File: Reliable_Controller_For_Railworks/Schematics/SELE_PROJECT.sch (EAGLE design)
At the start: 21 parts, among them IC1 24LC1025, IC2 MAX232, U1 328P, U2 LTC485N, U3 LTC485N, X1 16MHz

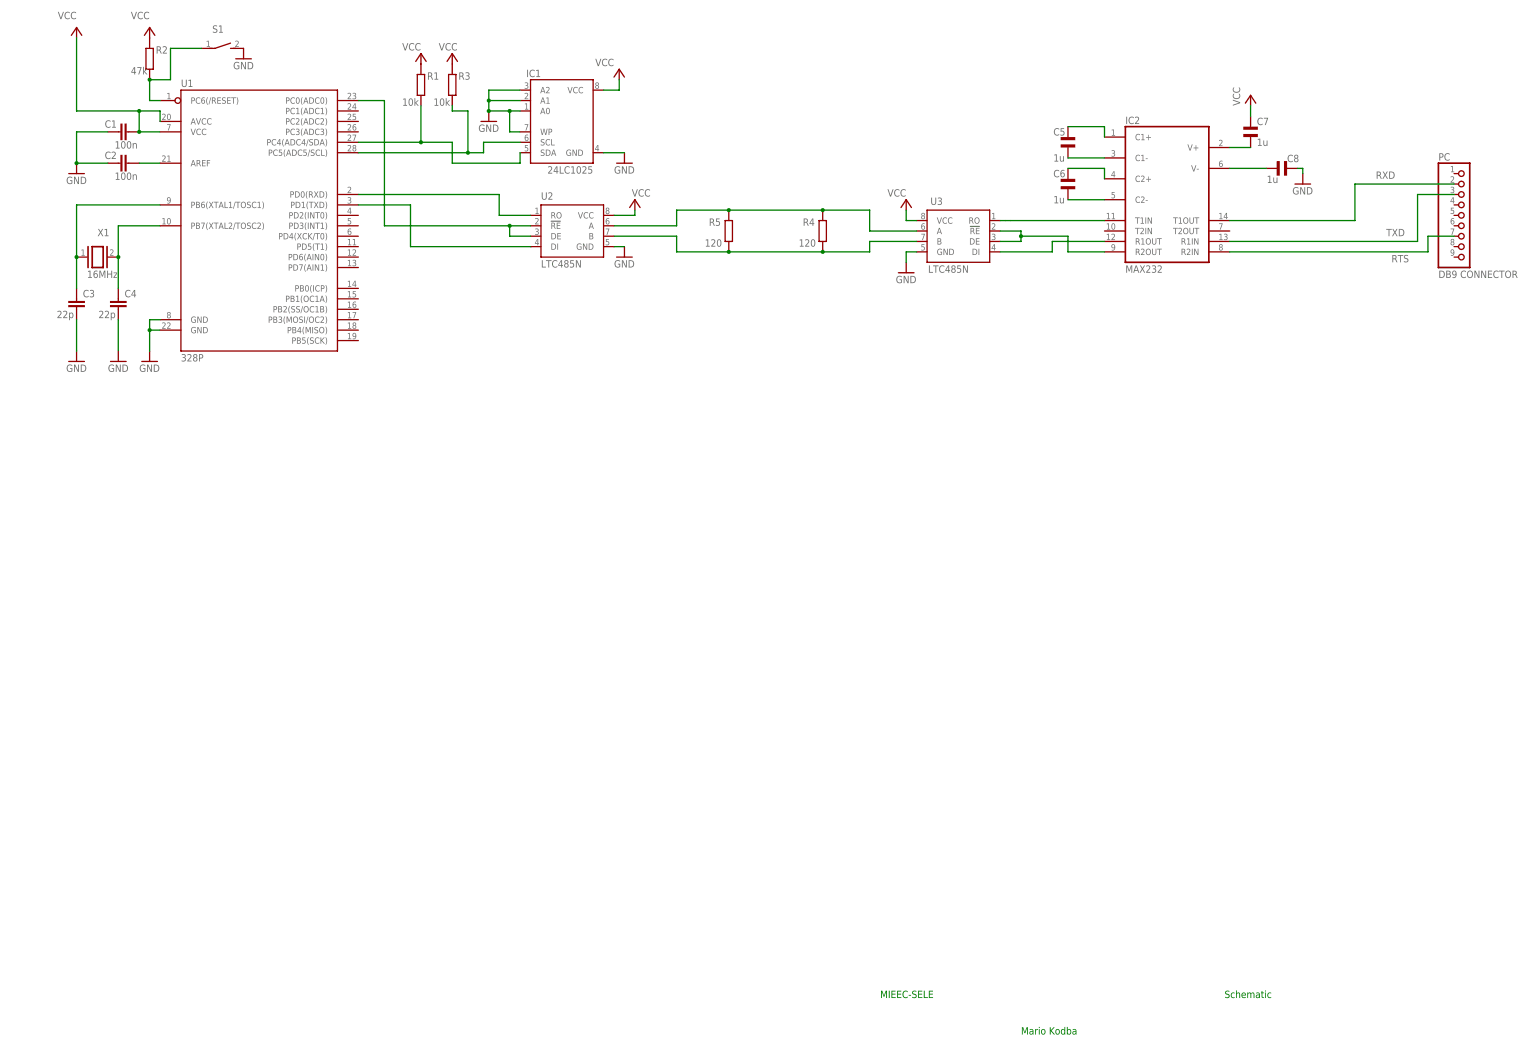
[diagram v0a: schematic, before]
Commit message: updated electrical schematic
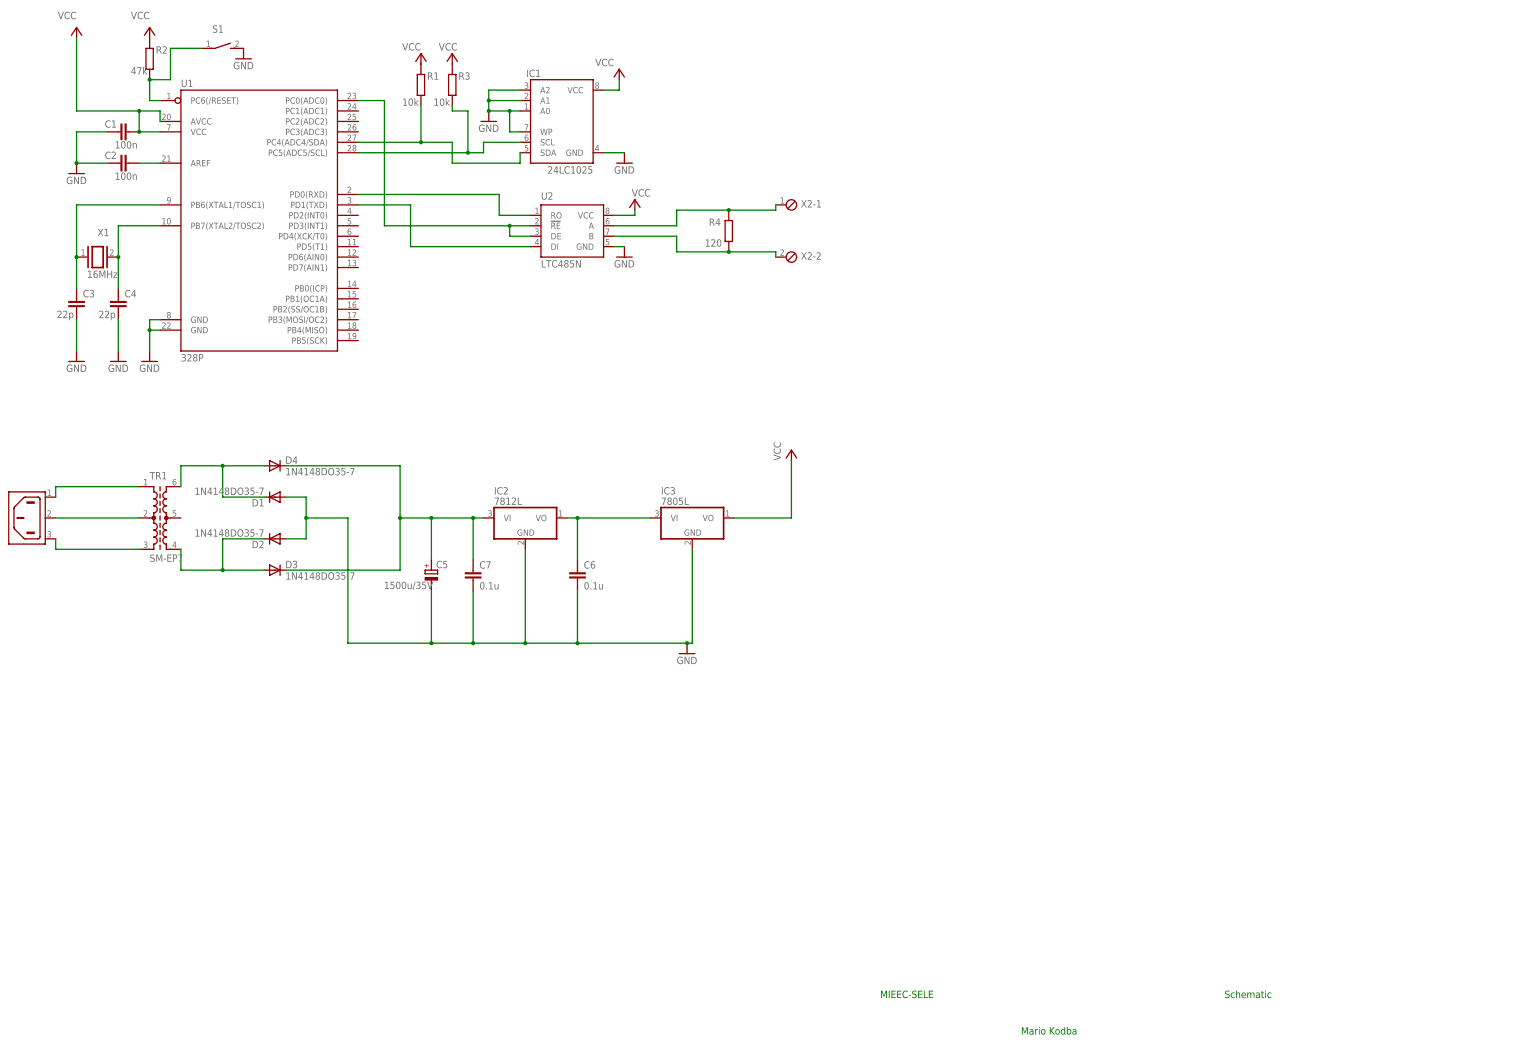
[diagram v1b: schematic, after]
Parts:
- removed C8: 1u, rcl:EL-BI25-10AXIAL
- removed PC: DB9 CONNECTOR, pinhead:PINHD-1X9
- removed R5: 120, eagle-ltspice:R
- removed U3: LTC485N, linear-technology:LTC485N
- added D1, D2, D3, D4: 1N4148DO35-7, diode:1N4148DO35-7
- added IC3: 7805L, linear:7805L
- added TR1: SM-EP7, inductor-neosid:SM-EP7
- added X2: (no value), con-phoenix-254:MPT2
- added X4: 6ESRM-P, con-tycoelectronics:6ESRM-P
- C5: value 1u -> 1500u/35V; device rcl:EL-BI25-10AXIAL -> rcl:CPOL-EU150CLZ-1010
- C6, C7: value 1u -> 0.1u; device rcl:EL-BI25-10AXIAL -> eagle-ltspice:CC1210
- IC2: value MAX232 -> 7812L; device maxim:MAX232 -> linear:7812L
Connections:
- removed net N$15: C6.2, IC2G$1.C2-
- removed net N$19: C8.2, IC2G$1.V-
- removed net RTS: IC2G$1.R2IN, PC.7
- removed net RXD: IC2G$1.T1OUT, PC.2
- removed net TXD: IC2G$1.R1IN, PC.3
- net GND: now also C5.-, C6.2, C7.2, D1.A, D2.A, IC2.GND, IC3.GND; no longer C8.1, U3.GND
- net N$11: now also D1.C, D4.A, TR1.6; no longer IC2G$1.T1IN, U3.RO
- net N$12: now also D2.C, D3.A, TR1.4; no longer IC2G$1.R1OUT, U3.DI
- net N$13: now also TR1.1, X4.AC1; no longer IC2G$1.R2OUT, U3.!RE, U3.DE
- net N$14: now also TR1.3, X4.AC2; no longer C5.1, IC2G$1.C1+
- net N$16: now also C5.+, C7.1, D3.C, D4.C, IC2.VI; no longer C6.1, IC2G$1.C2+
- net N$17: now also TR1.2, X4.SH; no longer C5.2, IC2G$1.C1-
- net N$18: now also C6.1, IC2.VO, IC3.VI; no longer C7.2, IC2G$1.V+
- net N$6: now also X2-1.1; no longer R5.1, U3.A
- net N$9: now also X2-2.1; no longer R5.2, U3.B
- net VCC: now also IC3.VO; no longer C7.1, U3.VCC
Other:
- moved on the sheet: R4
